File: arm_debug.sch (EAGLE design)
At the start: 11 parts

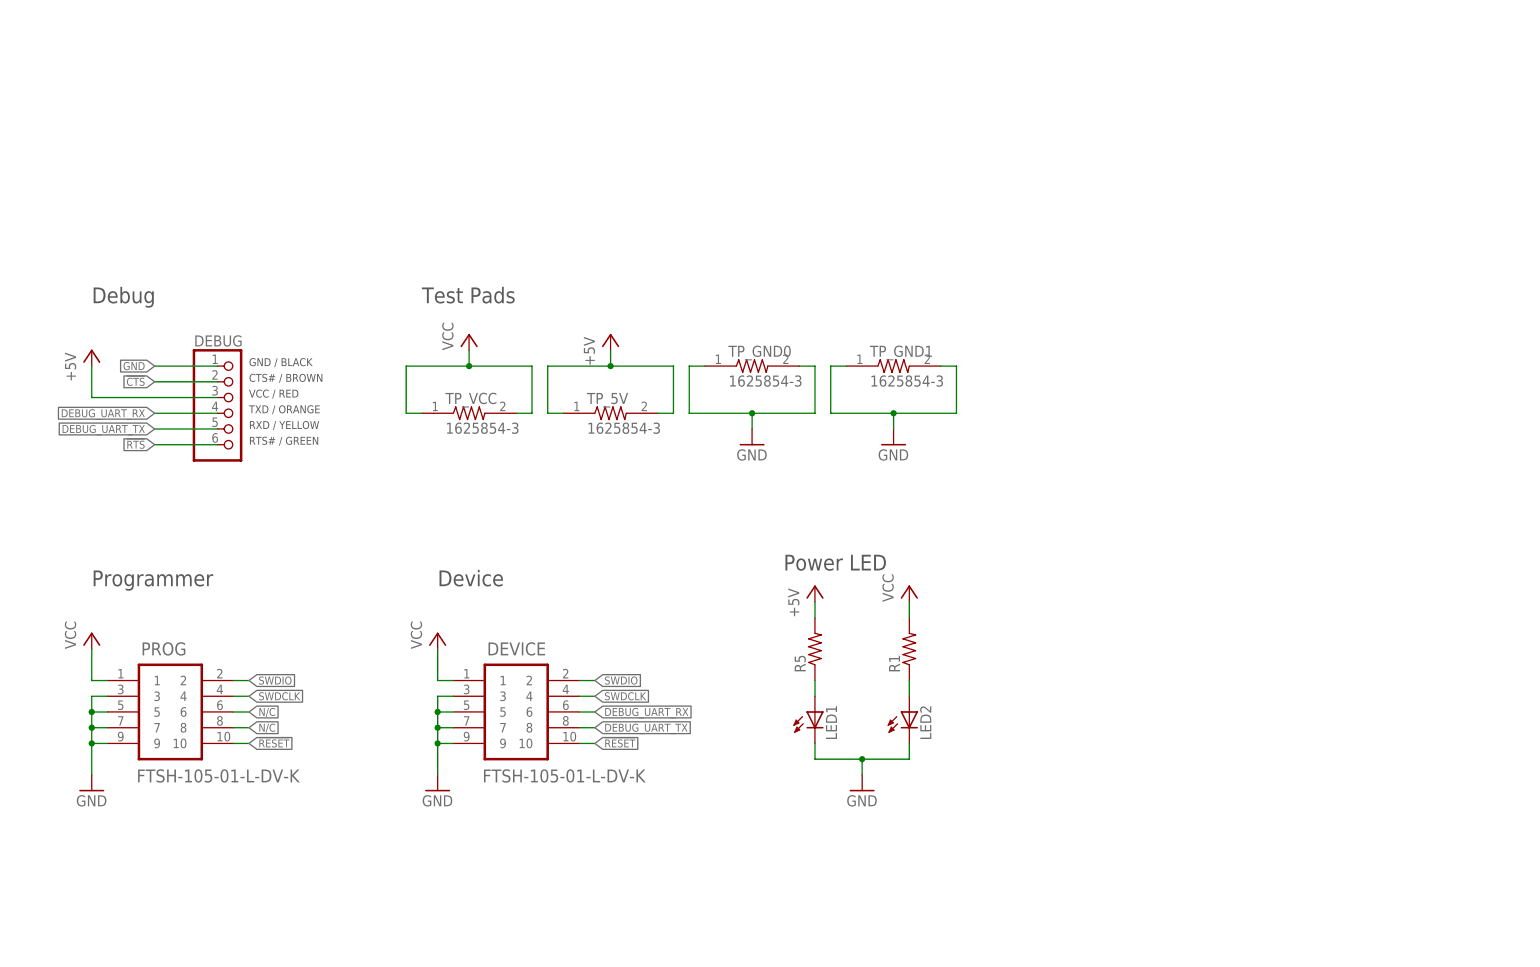
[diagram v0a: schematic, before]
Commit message: Saving place.. currently working on Rev B
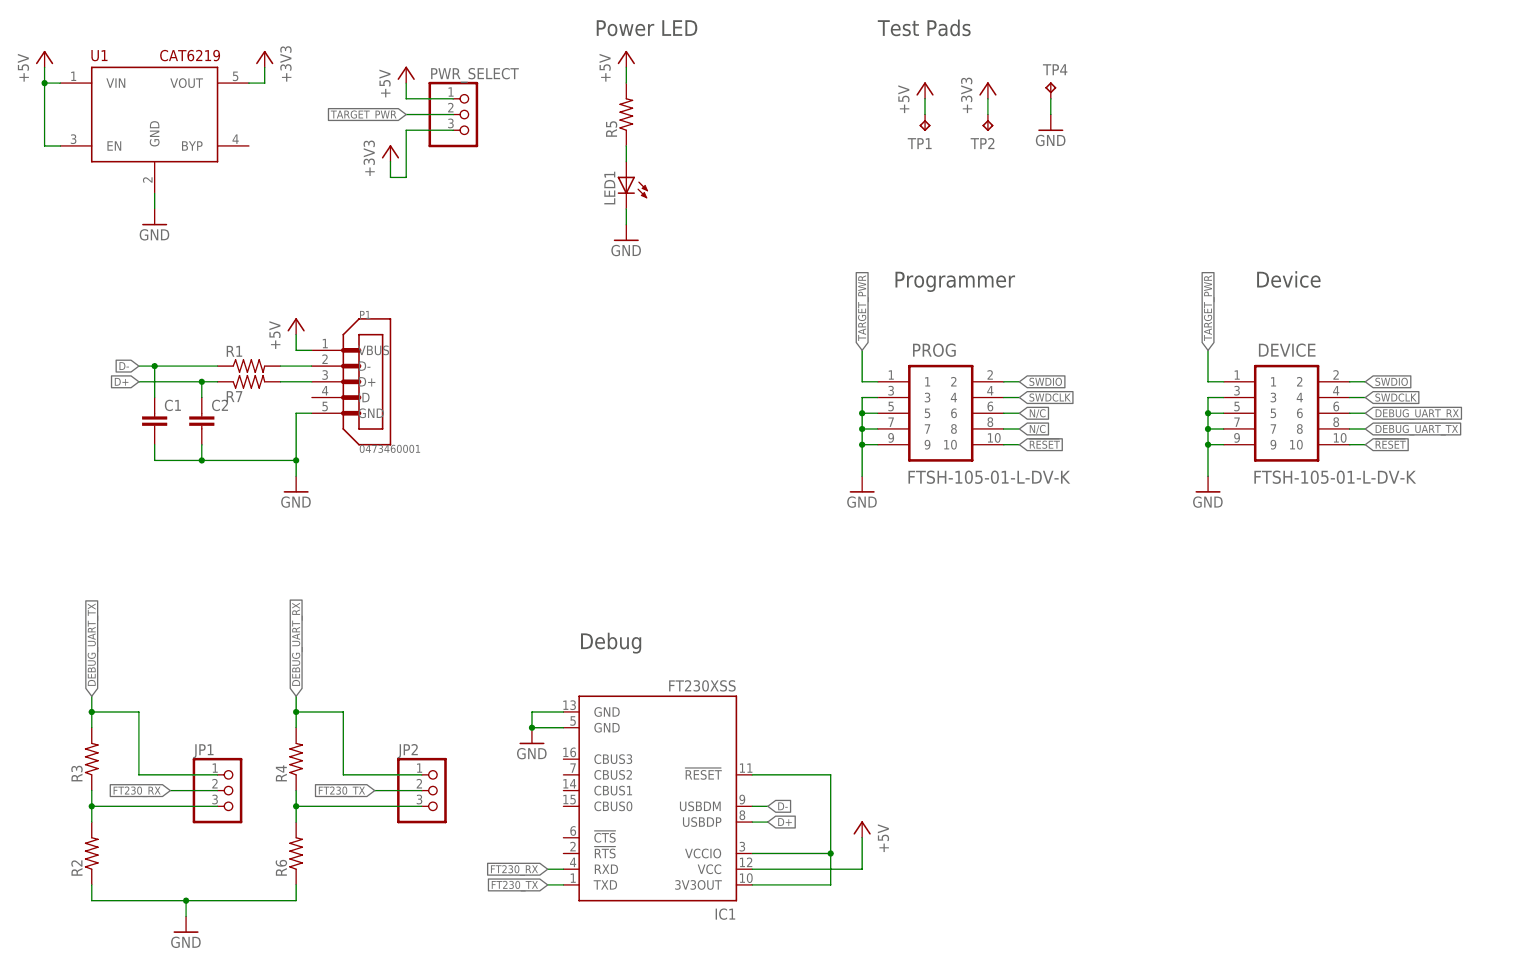
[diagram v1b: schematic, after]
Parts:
- removed DEBUG: (no value), pinhead:PINHD-1X6
- removed LED2: (no value), led:LEDSML0805
- removed TP_5V, TP_GND0, TP_GND1, TP_VCC: 1625854-3, 1625854-3:1625854-3
- added C1, C2: (no value), resistor:C-EUC0805
- added IC1: FT230XSS, FT230XS:FT230XSS
- added JP1, JP2, PWR_SELECT: (no value), pinhead:PINHD-1X3
- added P1: 0473460001, 0473460001:0473460001
- added R2, R3, R4, R6, R7: (no value), resistor:R-US_R0805
- added TP1, TP2, TP4: TPTP20SQ, testpad:TPTP20SQ
- added U1: CAT6219, CAT6219-330TDGT3:CAT6219
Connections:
- removed net !CTS: DEBUG.2
- removed net !RTS: DEBUG.6
- removed net VCC: DEVICE.1, PROG.1, R1.2, TP_VCC.1, TP_VCC.2
- new net +3V3: PWR_SELECT.3, TP2.TP, U1.VOUT
- new net D+: C2.1, IC1.USBDP, R7.1
- new net D-: C1.1, IC1.USBDM, R1.1
- new net FT230_RX: IC1.RXD, JP1.2
- new net FT230_TX: IC1.TXD, JP2.2
- new net N$3: IC1.!RESET, IC1.3V3OUT, IC1.VCCIO
- new net N$4: P1.D+, R7.2
- new net N$7: JP2.3, R4.1, R6.2
- new net N$8: JP1.3, R2.2, R3.1
- new net TARGET_PWR: DEVICE.1, PROG.1, PWR_SELECT.2
- net +5V: now also IC1.VCC, P1.VBUS, PWR_SELECT.1, TP1.TP, U1.EN, U1.VIN; no longer DEBUG.3, TP_5V.1, TP_5V.2
- net DEBUG_UART_RX: now also JP2.1, R4.2; no longer DEBUG.4
- net DEBUG_UART_TX: now also JP1.1, R3.2; no longer DEBUG.5
- net GND: now also C1.2, C2.2, IC1.GND, IC1.GND@1, P1.GND, R2.1, R6.1, TP4.TP, U1.GND; no longer DEBUG.1, LED2.C, TP_GND0.1, TP_GND0.2, TP_GND1.1, TP_GND1.2
- net N$2: now also P1.D-, R1.2; no longer LED2.A, R1.1
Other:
- note removed: "CTS# / BROWN"
- note removed: "GND / BLACK"
- note removed: "RTS# / GREEN"
- note removed: "RXD / YELLOW"
- note removed: "TXD / ORANGE"
- note removed: "VCC / RED"
- moved on the sheet: DEVICE, LED1, PROG, R1, R5

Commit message: Committing RevB
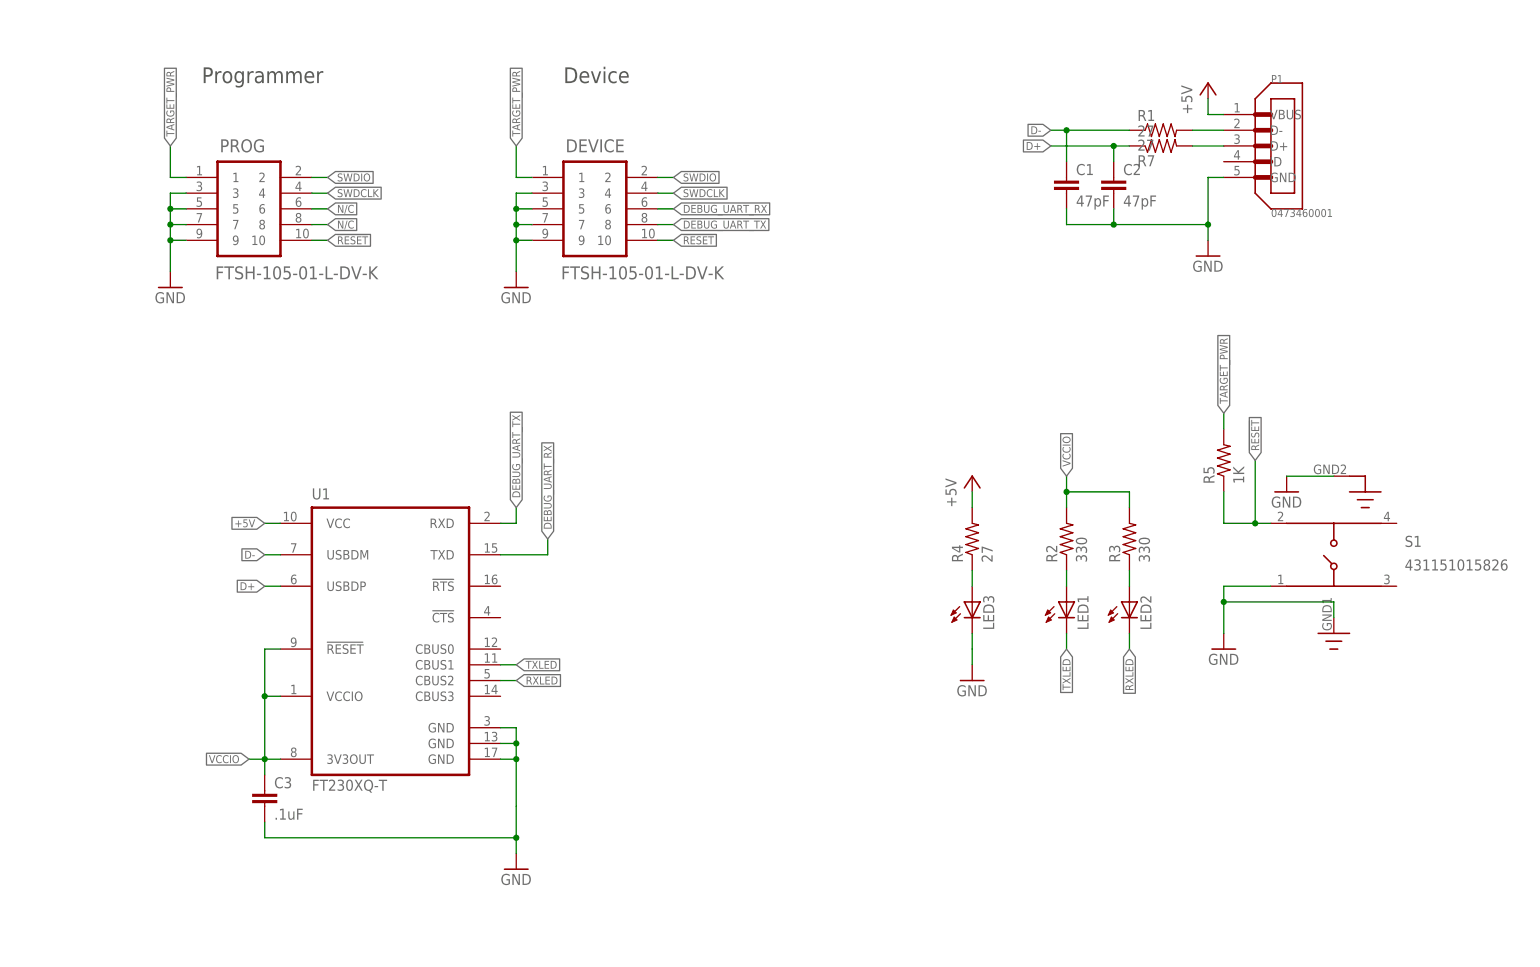
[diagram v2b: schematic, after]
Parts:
- removed IC1: FT230XSS, FT230XS:FT230XSS
- removed JP1, JP2, PWR_SELECT: (no value), pinhead:PINHD-1X3
- removed R6: (no value), resistor:R-US_R0805
- removed TP1, TP2, TP4: TPTP20SQ, testpad:TPTP20SQ
- added C3: .1uF, resistor:C-EUC0603
- added LED2, LED3: (no value), led:LEDCHIPLED_0603
- added S1: 431151015826, 431151015826:431151015826
- C1, C2: value (none) -> 47pF; device resistor:C-EUC0805 -> resistor:C-EUC0603
- LED1: device led:LEDSML0805 -> led:LEDCHIPLED_0603
- R1, R4, R7: value (none) -> 27; device resistor:R-US_R0805 -> resistor:R-US_R0603
- R2, R3: value (none) -> 330; device resistor:R-US_R0805 -> resistor:R-US_R0603
- R5: value (none) -> 1K; device resistor:R-US_R0805 -> resistor:R-US_R0603
- U1: value CAT6219 -> FT230XQ-T; device CAT6219-330TDGT3:CAT6219 -> FT230XQ-T:FT230XQ-T
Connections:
- removed net +3V3: PWR_SELECT.3, TP2.TP, U1.VOUT
- removed net FT230_RX: IC1.RXD, JP1.2
- removed net FT230_TX: IC1.TXD, JP2.2
- removed net N$1: LED1.A, R5.1
- removed net N$7: JP2.3, R4.1, R6.2
- removed net N$8: JP1.3, R2.2, R3.1
- new net N$14: LED1.A, R2.1
- new net N$9: LED2.A, R3.1
- new net RXLED: LED2.C, U1.CBUS2
- new net TXLED: LED1.C, U1.CBUS1
- new net VCCIO: C3.1, R2.2, R3.2, U1.!RESET!, U1.3V3OUT, U1.VCCIO
- net !RESET: now also R5.1, S1.2
- net +5V: now also R4.2, U1.VCC; no longer IC1.VCC, PWR_SELECT.1, R5.2, TP1.TP, U1.EN, U1.VIN
- net D+: now also U1.USBDP; no longer IC1.USBDP
- net D-: now also U1.USBDM; no longer IC1.USBDM
- net DEBUG_UART_RX: now also U1.TXD; no longer JP2.1, R4.2
- net DEBUG_UART_TX: now also U1.RXD; no longer JP1.1, R3.2
- net GND: now also C3.2, LED3.C, S1.1, S1.5, S1.6, U1.GND@13, U1.GND@17, U1.GND@3; no longer IC1.GND, IC1.GND@1, LED1.C, R2.1, R6.1, TP4.TP, U1.GND
- net N$3: now also LED3.A, R4.1; no longer IC1.!RESET, IC1.3V3OUT, IC1.VCCIO
- net TARGET_PWR: now also R5.2; no longer PWR_SELECT.2
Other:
- note removed: "Debug"
- note removed: "Power LED"
- note removed: "Test Pads"
- moved on the sheet: C1, C2, DEVICE, LED1, P1, PROG, R1, R2, R3, R4, R5, R7

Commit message: Commiting RevC
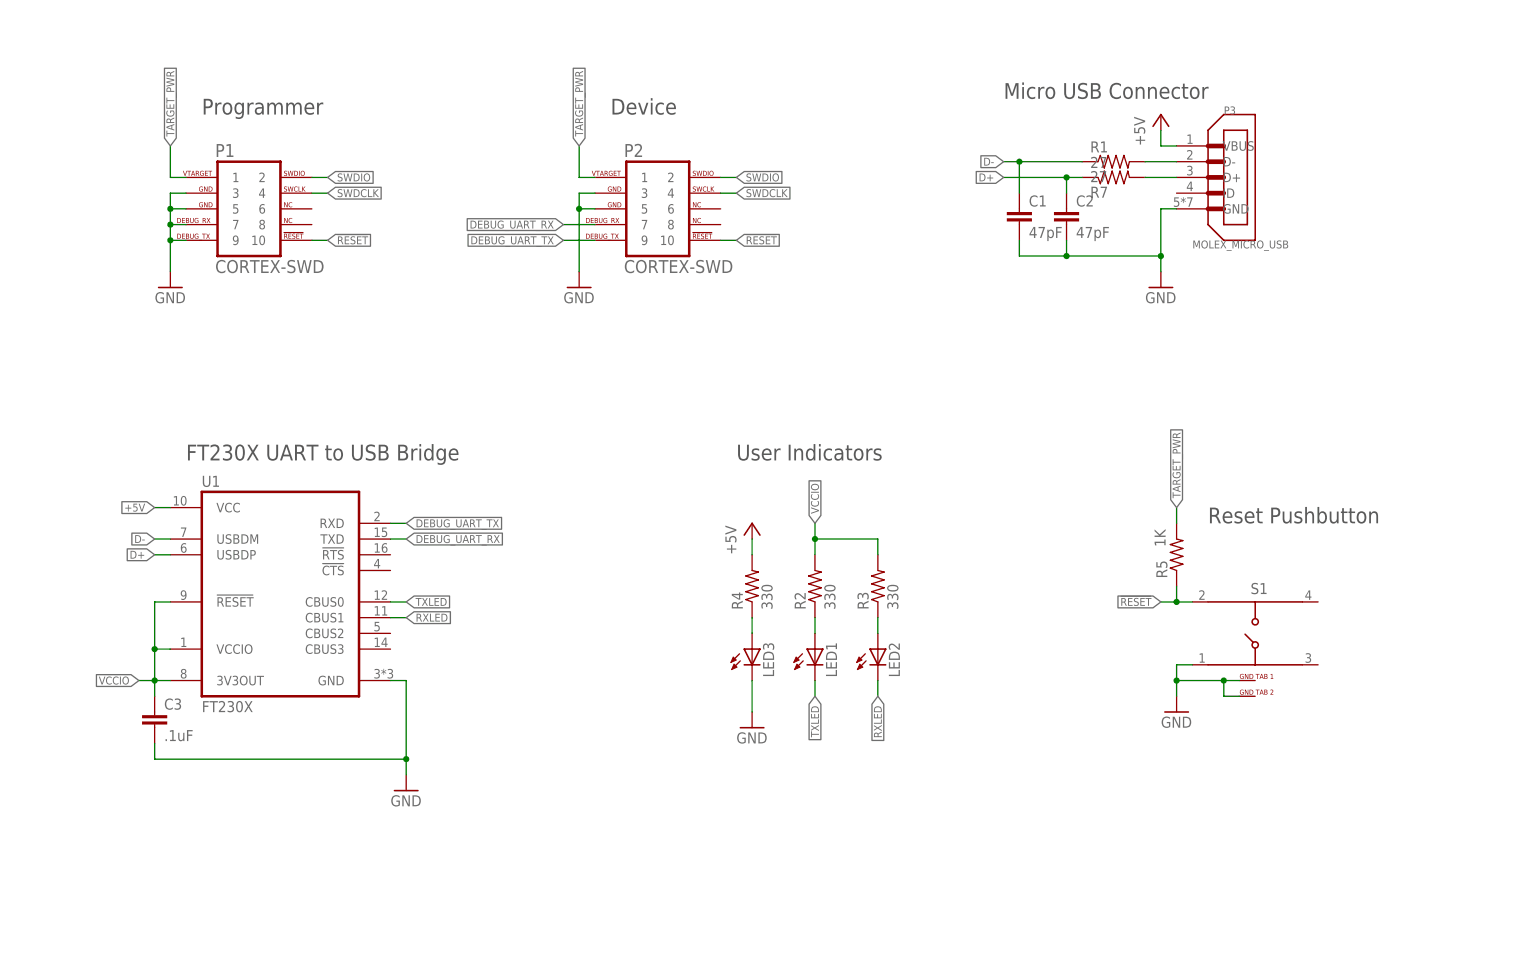
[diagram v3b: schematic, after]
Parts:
- removed DEVICE, PROG: FTSH-105-01-L-DV-K, FTSH-105-01-L-DV-K:FTSH-105-01-L-DV-K
- added P2: CORTEX-SWD, programming_headers:SWD-CORTEX
- added P3: MOLEX_MICRO_USB, board_connectivity:MOLEX_MICRO_USB
- P1: value 0473460001 -> CORTEX-SWD; device 0473460001:0473460001 -> programming_headers:SWD-CORTEX
- R4: value 27 -> 330
- S1: value 431151015826 -> WURTH_SMD_PB; device 431151015826:431151015826 -> switches:WURTH_SMD_PB
- U1: value FT230XQ-T -> FT230X; device FT230XQ-T:FT230XQ-T -> USB:FT230XQ
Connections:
- removed net N/C: PROG.6, PROG.8
- net !RESET: now also P1.10, P2.10; no longer DEVICE.10, PROG.10
- net +5V: now also P3.VBUS; no longer P1.VBUS
- net DEBUG_UART_RX: now also P2.7; no longer DEVICE.6
- net DEBUG_UART_TX: now also P2.9; no longer DEVICE.8
- net GND: now also P1.3, P1.5, P1.7, P1.9, P2.3, P2.5, P3.GND, U1.GND; no longer DEVICE.3, DEVICE.5, DEVICE.7, DEVICE.9, P1.GND, PROG.3, PROG.5, PROG.7, PROG.9, U1.GND@13, U1.GND@17, U1.GND@3
- net N$2: now also P3.D-; no longer P1.D-
- net N$4: now also P3.D+; no longer P1.D+
- net RXLED: now also U1.CBUS1; no longer U1.CBUS2
- net SWDCLK: now also P1.4, P2.4; no longer DEVICE.4, PROG.4
- net SWDIO: now also P1.2, P2.2; no longer DEVICE.2, PROG.2
- net TARGET_PWR: now also P1.1, P2.1; no longer DEVICE.1, PROG.1
- net TXLED: now also U1.CBUS0; no longer U1.CBUS1
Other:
- note added: "FT230X UART to USB Bridge"
- note added: "Micro USB Connector"
- note added: "Reset Pushbutton"
- note added: "User Indicators"
- moved on the sheet: C1, C2, C3, LED1, LED2, LED3, R1, R2, R3, R4, R5, R7
